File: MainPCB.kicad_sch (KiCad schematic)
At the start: 57 parts, among them J1 RaspberryPi, J2 Conn_01x05, J3 Screw_Terminal_01x02, J4 Conn_01x02, J5 Conn_01x06, J6 Conn_01x03_Pin, J7 Conn_01x05, J8 Conn_01x12, M1 Motor_DC, M2 Motor_DC, M3 Motor_DC, M4 Motor_DC, M5 Motor_DC, SW1 SW_SPDT, SW2 SW_SPDT, SW3 SW_SPDT, SW4 SW_SPDT, U1 Teensy4.1, U10 Compass, U11 V_Regulator5v, U12 RockerSwitch, U13 V_Regulator3.3v, U2 VNH Driver, U3 VNH Driver, U4 VNH Driver, U5 VNH Driver, U6 TSOP25xx, U7 V_Regulator5v, U8 VNH Driver

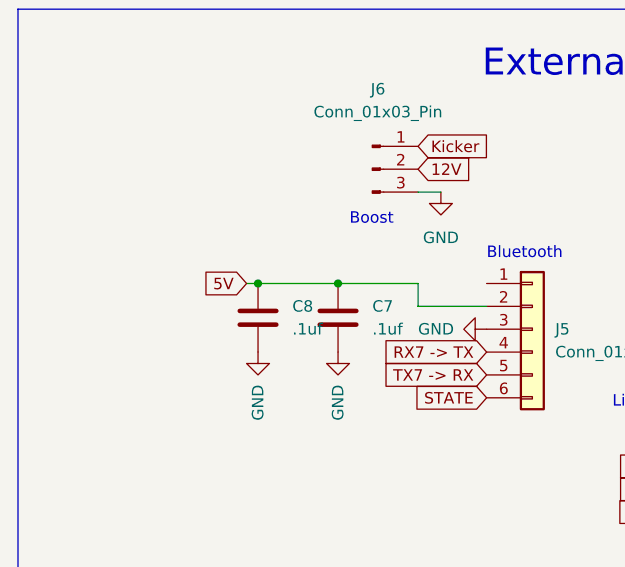
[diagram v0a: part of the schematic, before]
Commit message: moved stuff
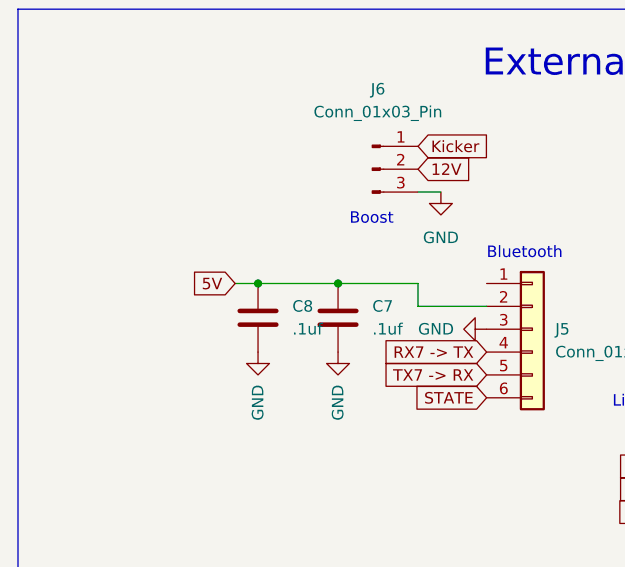
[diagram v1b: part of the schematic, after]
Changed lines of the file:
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@@
 	(wire
 		(pts
-			(xy 39.37 228.6) (xy 40.64 228.6)
+			(xy 38.1 228.6) (xy 40.64 228.6)
 		)
 		(stroke
@@
 	(global_label "5V"
 		(shape input)
-		(at 39.37 228.6 180)
-		(fields_autoplaced yes)
-		(effects
-			(font
-				(size 1.27 1.27)
-			)
-			(justify right)
-		)
-		(property "Intersheetrefs" "${INTERSHEET_REFS}"
-			(at 34.0867 228.6 0)
-			(effects
-				(font
+		(at 38.1 228.6 180)
+		(fields_autoplaced yes)
+		(effects
+			(font
+				(size 1.27 1.27)
+			)
+			(justify right)
+		)
+		(property "Intersheetrefs" "${INTERSHEET_REFS}"
+			(at 32.8167 228.6 0)
+			(effects
+				(font
